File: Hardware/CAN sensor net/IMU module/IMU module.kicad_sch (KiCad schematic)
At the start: 52 parts, among them SW1 SW_Push, SW2 SW_SPDT, U1 SN65HVD230, U2 STM32F103C8Tx, U3 W25Q32FVSSIG, Y1 16MHz

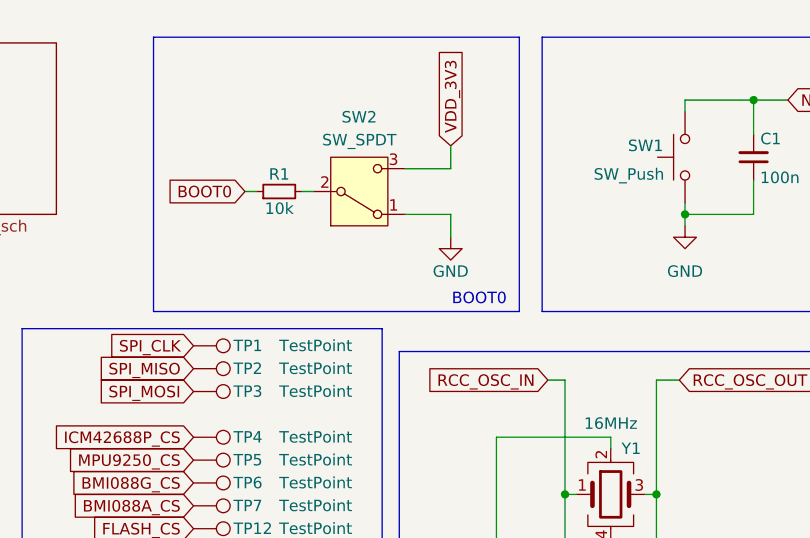
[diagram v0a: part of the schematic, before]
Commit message: IMU update
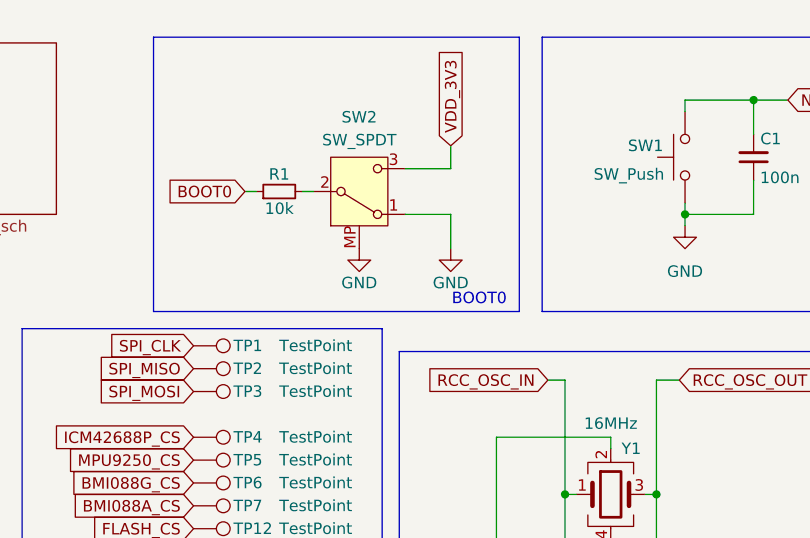
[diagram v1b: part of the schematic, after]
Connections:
- net GND: now also SW2.MP
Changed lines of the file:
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@@
 	(wire
 		(pts
-			(xy 142.875 37.465) (xy 142.875 40.005)
+			(xy 142.875 37.465) (xy 142.875 41.275)
 		)
 		(stroke
@@
 		(pin "1"
 		)
+		(pin "MP"
+		)
 		(instances
 			(project "IMU module"
@@
 		(lib_name "GND_1")
 		(lib_id "power:GND")
-		(at 142.875 40.005 0)
+		(at 142.875 41.275 0)
 		(unit 1)
 		(exclude_from_sim no)
@@
 		(dnp no)
 		(property "Reference" "#PWR02"
-			(at 142.875 46.355 0)
+			(at 142.875 47.625 0)
 			(effects
 				(font
@@
 		)
 		(property "Value" "GND"
-			(at 142.875 43.815 0)
+			(at 142.875 45.085 0)
 			(effects
 				(font
@@
 		)
 		(property "Footprint" ""
-			(at 142.875 40.005 0)
+			(at 142.875 41.275 0)
 			(effects
 				(font
@@
 		)
 		(property "Datasheet" ""
-			(at 142.875 40.005 0)
+			(at 142.875 41.275 0)
 			(effects
 				(font
@@
 		)
 		(property "Description" "Power symbol creates a global label with name \"GND\" , ground"
-			(at 142.875 40.005 0)
+			(at 142.875 41.275 0)
 			(effects
 				(font
@@
 					(unit 1)
 				)
+			)
+		)
+	)
+	(symbol
+		(lib_name "GND_1")
+		(lib_id "power:GND")
+		(at 132.715 41.275 0)
+		(unit 1)
+		(exclude_from_sim no)
+		(in_bom yes)
+		(on_board yes)
+		(dnp no)
+		(property "Reference" "#PWR026"
+			(at 132.715 47.625 0)
+			(effects
+				(font
+					(size 1.27 1.27)
+				)
+				(hide yes)
+			)
+		)
+		(property "Value" "GND"
+			(at 132.715 45.085 0)
+			(effects
+				(font
+					(size 1.27 1.27)
+				)
+			)
+		)
+		(property "Footprint" ""
+			(at 132.715 41.275 0)
+			(effects
+				(font
+					(size 1.27 1.27)
+				)
+				(hide yes)
+			)
+		)
+		(property "Datasheet" ""
+			(at 132.715 41.275 0)
+			(effects
+				(font
+					(size 1.27 1.27)
+				)
+				(hide yes)
+			)
+		)
+		(property "Description" "Power symbol creates a global label with name \"GND\" , ground"
+			(at 132.715 41.275 0)
+			(effects
+				(font
+					(size 1.27 1.27)
+				)
+				(hide yes)
+			)
+		)
+		(pin "1"
+		)
+		(instances
+			(project "IMU module"
+				(path "/62238c1b-6f7a-4963-9d99-86e391606da3"
+					(reference "#PWR026")
+					(unit 1)
+				)

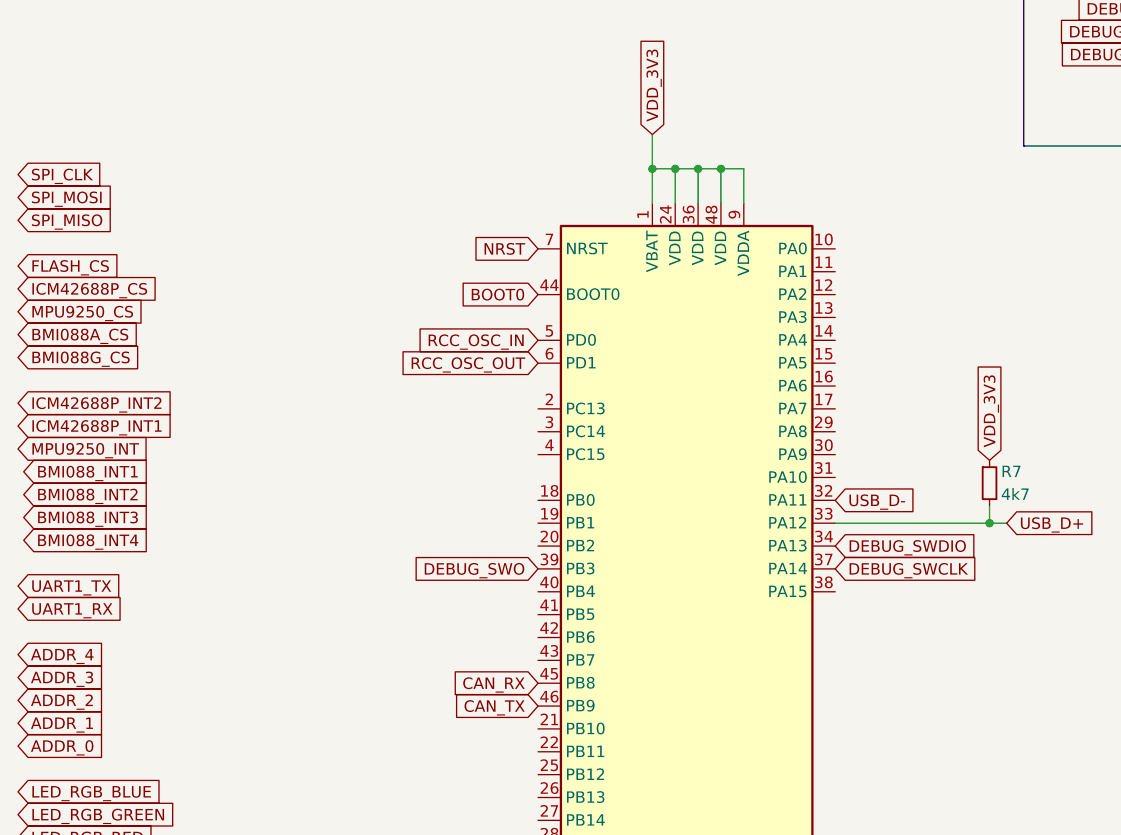
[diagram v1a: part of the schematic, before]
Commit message: Update IMU
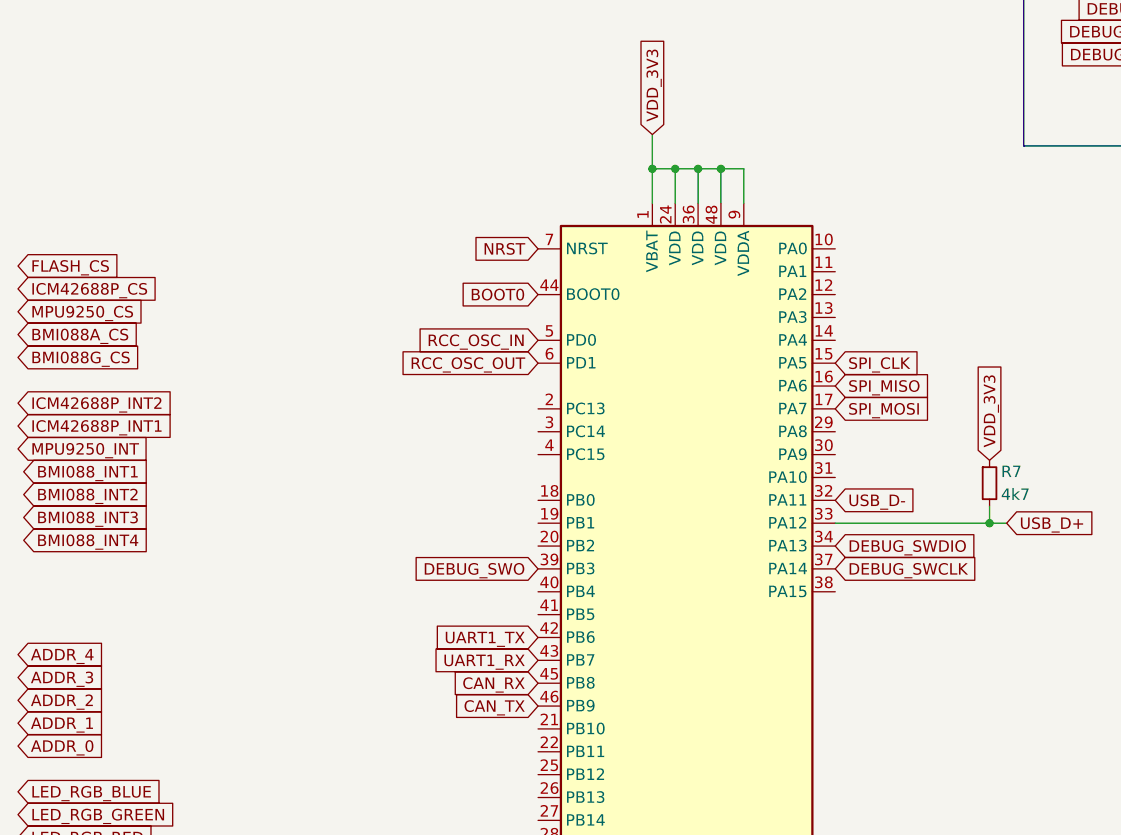
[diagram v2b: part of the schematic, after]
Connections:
- net SPI_CLK: now also U2.15 (PA5)
- net SPI_MISO: now also U2.16 (PA6)
- net SPI_MOSI: now also U2.17 (PA7)
- net UART1_RX: now also U2.43 (PB7)
- net UART1_TX: now also U2.42 (PB6)
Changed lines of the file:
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@@
 	(global_label "SPI_MOSI"
 		(shape input)
-		(at -16.51 98.425 0)
-		(fields_autoplaced yes)
-		(effects
-			(font
-				(size 1.27 1.27)
-			)
-			(justify left)
-		)
-		(property "Intersheetrefs" "${INTERSHEET_REFS}"
-			(at -4.8767 98.425 0)
+		(at 74.295 121.92 0)
+		(fields_autoplaced yes)
+		(effects
+			(font
+				(size 1.27 1.27)
+			)
+			(justify left)
+		)
+		(property "Intersheetrefs" "${INTERSHEET_REFS}"
+			(at 85.9283 121.92 0)
 			(effects
 				(font
@@
 	(global_label "SPI_MISO"
 		(shape input)
-		(at -16.51 100.965 0)
-		(fields_autoplaced yes)
-		(effects
-			(font
-				(size 1.27 1.27)
-			)
-			(justify left)
-		)
-		(property "Intersheetrefs" "${INTERSHEET_REFS}"
-			(at -4.8767 100.965 0)
+		(at 74.295 119.38 0)
+		(fields_autoplaced yes)
+		(effects
+			(font
+				(size 1.27 1.27)
+			)
+			(justify left)
+		)
+		(property "Intersheetrefs" "${INTERSHEET_REFS}"
+			(at 85.9283 119.38 0)
 			(effects
 				(font
@@
 	(global_label "UART1_RX"
 		(shape input)
-		(at -16.51 144.145 0)
-		(fields_autoplaced yes)
-		(effects
-			(font
-				(size 1.27 1.27)
-			)
-			(justify left)
-		)
-		(property "Intersheetrefs" "${INTERSHEET_REFS}"
-			(at -4.2115 144.145 0)
-			(effects
-				(font
-					(size 1.27 1.27)
-				)
-				(justify left)
+		(at 41.275 149.86 180)
+		(fields_autoplaced yes)
+		(effects
+			(font
+				(size 1.27 1.27)
+			)
+			(justify right)
+		)
+		(property "Intersheetrefs" "${INTERSHEET_REFS}"
+			(at 28.9765 149.86 0)
+			(effects
+				(font
+					(size 1.27 1.27)
+				)
+				(justify right)
 				(hide yes)
 			)
@@
 	(global_label "SPI_CLK"
 		(shape input)
-		(at -16.51 95.885 0)
-		(fields_autoplaced yes)
-		(effects
-			(font
-				(size 1.27 1.27)
-			)
-			(justify left)
-		)
-		(property "Intersheetrefs" "${INTERSHEET_REFS}"
-			(at -5.9048 95.885 0)
+		(at 74.295 116.84 0)
+		(fields_autoplaced yes)
+		(effects
+			(font
+				(size 1.27 1.27)
+			)
+			(justify left)
+		)
+		(property "Intersheetrefs" "${INTERSHEET_REFS}"
+			(at 84.9002 116.84 0)
 			(effects
 				(font
@@
 	(global_label "UART1_TX"
 		(shape input)
-		(at -16.51 141.605 0)
-		(fields_autoplaced yes)
-		(effects
-			(font
-				(size 1.27 1.27)
-			)
-			(justify left)
-		)
-		(property "Intersheetrefs" "${INTERSHEET_REFS}"
-			(at -4.5139 141.605 0)
-			(effects
-				(font
-					(size 1.27 1.27)
-				)
-				(justify left)
-				(hide yes)
-			)
+		(at 41.275 147.32 180)
+		(fields_autoplaced yes)
+		(effects
+			(font
+				(size 1.27 1.27)
+			)
+			(justify right)
+		)
+		(property "Intersheetrefs" "${INTERSHEET_REFS}"
+			(at 29.2789 147.32 0)
+			(effects
+				(font
+					(size 1.27 1.27)
+				)
+				(justify right)
+				(hide yes)
+			)
